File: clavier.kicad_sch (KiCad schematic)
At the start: 0 parts

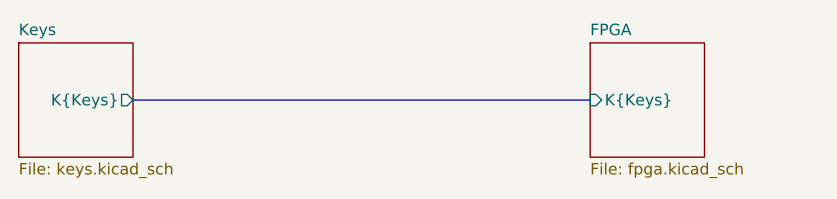
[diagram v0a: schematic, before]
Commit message: Initial commit of the PCB
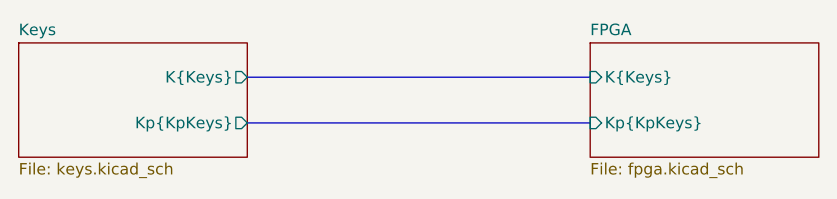
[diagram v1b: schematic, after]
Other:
- sheet FPGA ports: added Kp{KpKeys}; removed none
- sheet Keys ports: added Kp{KpKeys}; removed none
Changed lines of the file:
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@@
 	(bus
 		(pts
-			(xy 114.3 82.55) (xy 165.1 82.55)
+			(xy 127 80.01) (xy 165.1 80.01)
+		)
+		(stroke
+			(width 0)
+			(type default)
+		)
+	)
+	(bus
+		(pts
+			(xy 127 85.09) (xy 165.1 85.09)
 		)
 		(stroke
@@
 	(sheet
 		(at 165.1 76.2)
-		(size 12.7 12.7)
+		(size 25.4 12.7)
 		(exclude_from_sim no)
 		(in_bom yes)
@@
 		)
 		(pin "K{Keys}" input
-			(at 165.1 82.55 180)
+			(at 165.1 80.01 180)
+			(effects
+				(font
+					(size 1.27 1.27)
+				)
+				(justify left)
+			)
+		)
+		(pin "Kp{KpKeys}" input
+			(at 165.1 85.09 180)
 			(effects
 				(font
@@
 	(sheet
 		(at 101.6 76.2)
-		(size 12.7 12.7)
+		(size 25.4 12.7)
 		(exclude_from_sim no)
 		(in_bom yes)
@@
 			)
 		)
-		(pin "K{Keys}" output
-			(at 114.3 82.55 0)
+		(pin "Kp{KpKeys}" output
+			(at 127 85.09 0)
 			(effects
 				(font
+					(size 1.27 1.27)
+				)
+				(justify right)
+			)
+		)
+		(pin "K{Keys}" output
+			(at 127 80.01 0)
+			(effects
+				(font
